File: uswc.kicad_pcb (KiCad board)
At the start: 2 copper layers, 43.3 x 30 mm, 61 parts, among them J1 USB_C_Receptacle, J2 Conn_01x02_Socket, J3 Conn_01x08_Pin, P1 DFP, SW1 SW_SPDT, U10 SRV05-4, U13 LM2903, U2 W25Q32JVZP, U3 SN74LVC1T45DBV, U4 RP2040, U5 XC6206PxxxMR, U6 74LVC1G125, U7 LM397, U8 TS5A23166DCU, U9 SRV05-4, Y1 12MHz 10ppm, Y2 12MHz 10ppm

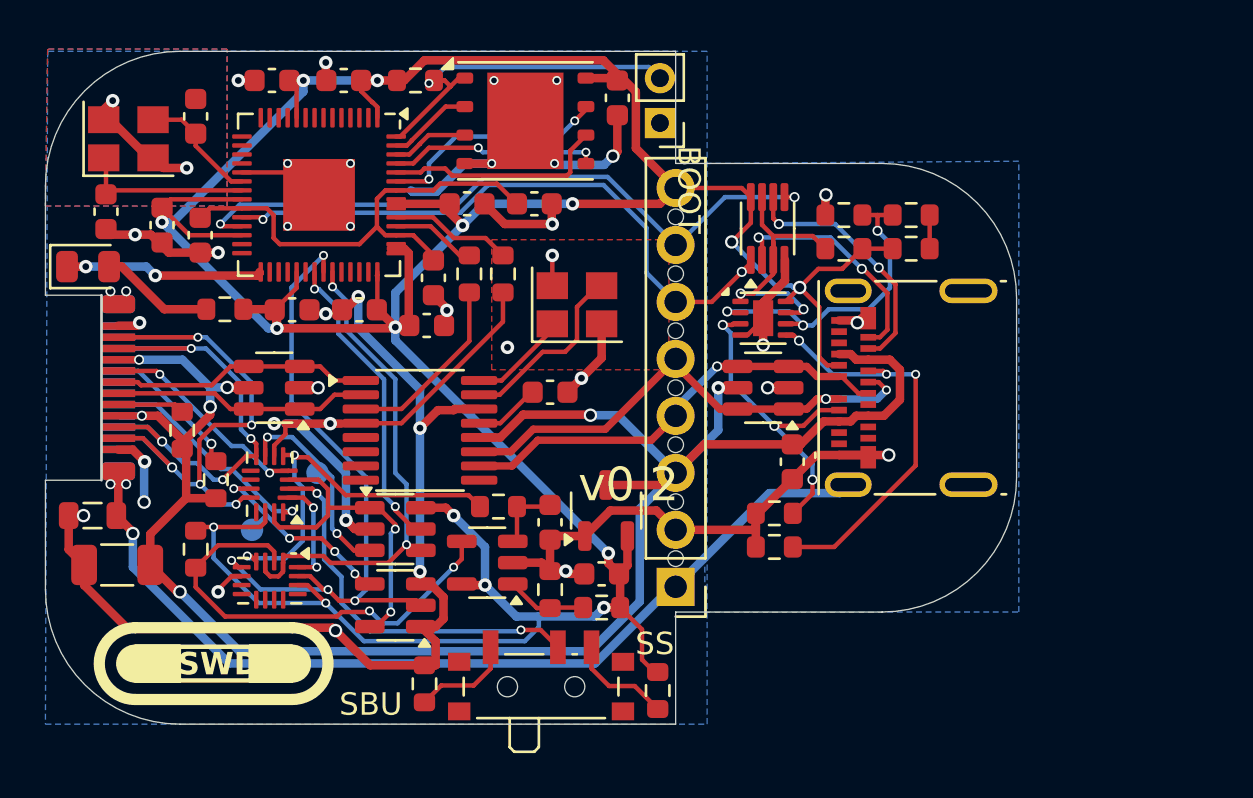
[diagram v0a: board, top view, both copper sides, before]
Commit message: backup
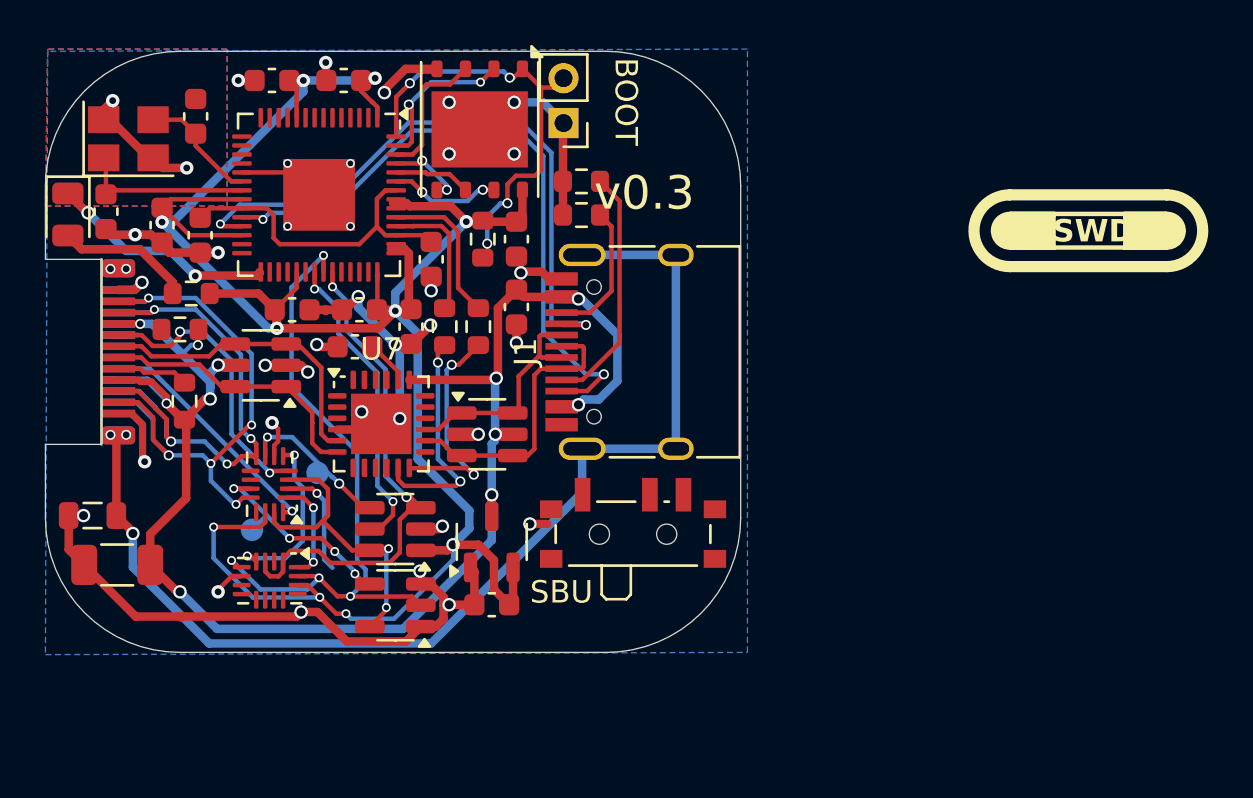
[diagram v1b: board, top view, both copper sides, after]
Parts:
- removed C2, C5: 1uF, Capacitor_SMD:C_0603_1608Metric
- removed C7: 0.1uF, Capacitor_SMD:C_0603_1608Metric
- removed J3: Conn_01x08_Pin, Connector_PinHeader_2.54mm:PinHeader_1x08_P2.54mm_Vertical
- removed R10, R12, R13, R16, R5, R6, R7: 56k, Resistor_SMD:R_0603_1608Metric
- removed R11, R22, R23: 5.1k, Resistor_SMD:R_0603_1608Metric
- removed REF**: header-bites, uswc:header-bites
- removed U1: ~, Package_SO:QSOP-16_3.9x4.9mm_P0.635mm
- removed U13: LM2903, Package_DFN_QFN:DFN-8-1EP_2x2mm_P0.5mm_EP0.9x1.6mm
- removed U8: TS5A23166DCU, Package_SO:VSSOP-8_2.3x2mm_P0.5mm
- removed Y1: 12MHz 10ppm, Crystal:Crystal_SMD_3225-4Pin_3.2x2.5mm
- J1: value USB_C_Receptacle -> USB_C_Receptacle_USB2.0_16P; footprint Connector_USB:USB_C_Receptacle_Molex_105450-0101 -> Connector_USB:USB_C_Receptacle_HRO_TYPE-C-31-M-12
- U7: value LM397 -> CH334F; footprint Package_TO_SOT_SMD:SOT-23-5 -> Package_DFN_QFN:QFN-24-1EP_4x4mm_P0.5mm_EP2.7x2.7mm
- moved R1 17.1 mm to (77.4, 109.8)
- moved R2 17.1 mm to (77.4, 111.3)
- moved C14 14.1 mm to (74.5, 115.4)
- moved U9 12.5 mm to (73.2, 121.1), turned to 0 degrees
- moved J1 11.7 mm to (80.6, 117.4)
- moved C1 8.93 mm to (67.3, 117.2), turned to 0 degrees
- moved SW1 7.94 mm to (79.7, 125.2)
- moved U7 7.79 mm to (68.5, 120.6), turned to 0 degrees
- moved C20 7.74 mm to (74.5, 112.4)
- moved R14 7.68 mm to (73.0, 112.4), turned to 90 degrees
- moved R9 6.89 mm to (59.5, 116.4), turned to 0 degrees
- moved U5 5.29 mm to (73.4, 125.9)
- moved C3 5.22 mm to (70.7, 113.3), turned to -90 degrees
- moved C19 5.09 mm to (73.4, 128.7)
- moved J2 4.30 mm to (76.6, 107.2)
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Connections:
- C1 pad 2: Net-(U1-VDD33) -> Net-(U7-VDD33)
- J1 pad A8: +3V3 -> DBG_SWD
- J1 pad B8: unconnected-(J1-SBU2-PadB8) -> DBG_SWC
- P1 pad A5: Net-(P1-CC) -> DFP_CC1
- P1 pad B5: Net-(P1-VCONN) -> DFP_CC2
- R8 pad 1: Net-(P1-CC) -> DFP_CC1
- R9 pad 1: Net-(P1-VCONN) -> DFP_CC2
- SW1 pad 1: Net-(SW1-A) -> GND
- SW1 pad 3: Net-(SW1-C) -> +3V3
- U3 pad 1: DUT_VREF -> +3V3
- U3 pad 3: DUT_SWD_L -> DUT_SWD
- U3 pad 4: DUT_SWD -> DUT_SWD_L
- U3 pad 6: +3V3 -> DUT_VREF
- U4 pad 34: unconnected-(U4-GPIO22-Pad34) -> DUT_SBU_SWD_ALT
- U4 pad 38: unconnected-(U4-GPIO26_ADC0-Pad38) -> DFP_CC1
- U4 pad 39: unconnected-(U4-GPIO27_ADC1-Pad39) -> DFP_CC2
- U4 pad 40: unconnected-(U4-GPIO28_ADC2-Pad40) -> DUT_SWD/C_SBU
- U4 pad 41: unconnected-(U4-GPIO29_ADC3-Pad41) -> DUT_SWC/D_SBU
- U7 pad 1: Net-(U7--) -> unconnected-(U7-~{OVCUR}-Pad1)
- U7 pad 2: GND -> unconnected-(U7-NC-Pad2)
- U7 pad 3: Net-(U7-+) -> unconnected-(U7-XO-Pad3)
- U7 pad 4: DUT_SBU_SWD_ALT -> GND
- U7 pad 5: +3V3 -> DUT_D-
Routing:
- net +3V3: track 168.7 -> 103.6 mm, vias 15 -> 10
- net GND: track 135.8 -> 86.7 mm, vias 40 -> 37
- net DUT_SBU_SWD_ALT: track 20.0 -> 0.00 mm, vias 2 -> 0
- net VBUS: track 85.9 -> 71.4 mm, vias 7 -> 11
- net Net-(U13A--): track 14.4 -> 0.00 mm, vias 3 -> 0
- net Net-(U8-IN1): track 13.1 -> 0.00 mm, vias 2 -> 0
- net CC2: track 18.7 -> 6.22 mm, vias 3 -> 0
- net D+: track 22.7 -> 10.2 mm, vias 2 -> 0
- net USE_SS: track 17.2 -> 4.95 mm, vias 2 -> 1
- net DBG_SWD_S: track 11.3 -> 0.00 mm, vias 2 -> 0
- net DBG_SWC_S: track 10.5 -> 0.00 mm, vias 2 -> 0
- net DUT_SWD/C_SBU: track 17.1 -> 7.84 mm
- net Net-(U1-XO): track 8.19 -> 0.00 mm
- net SHIELD: track 42.0 -> 50.1 mm
- net D-: track 19.5 -> 12.8 mm, vias 1 -> 0
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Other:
- board size 43.3 x 30 mm -> 31 x 26.8 mm
- board text added: "SB"
- board text added: "v0.3"
- board text removed: "SS"
- board text removed: "T2"
- board text removed: "v0.2"
